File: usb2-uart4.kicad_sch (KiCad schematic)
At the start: 14 parts, among them U1 FT4232H, U2 NUP2202, U3 93LCxxB, Y1 12.000 MHz

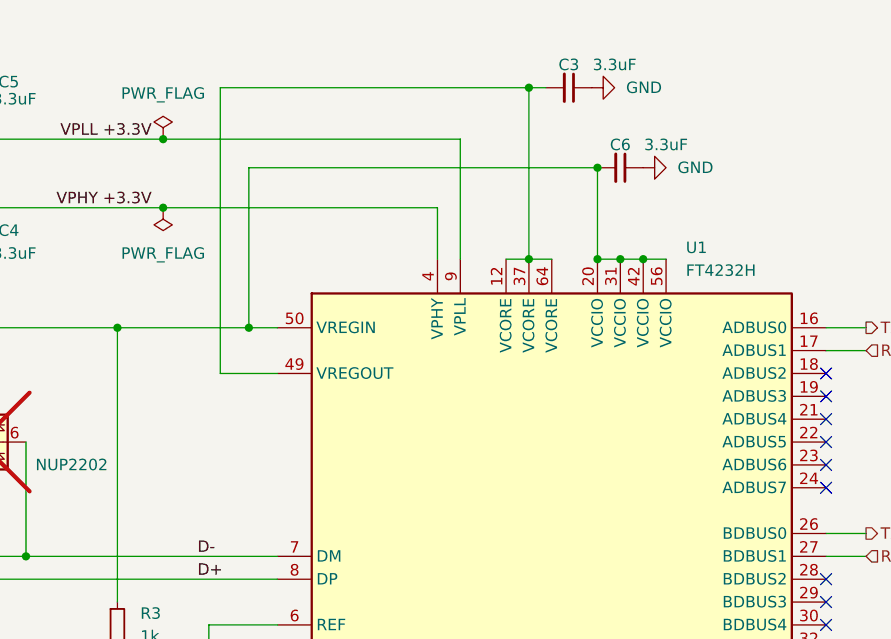
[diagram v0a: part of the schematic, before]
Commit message: Flush
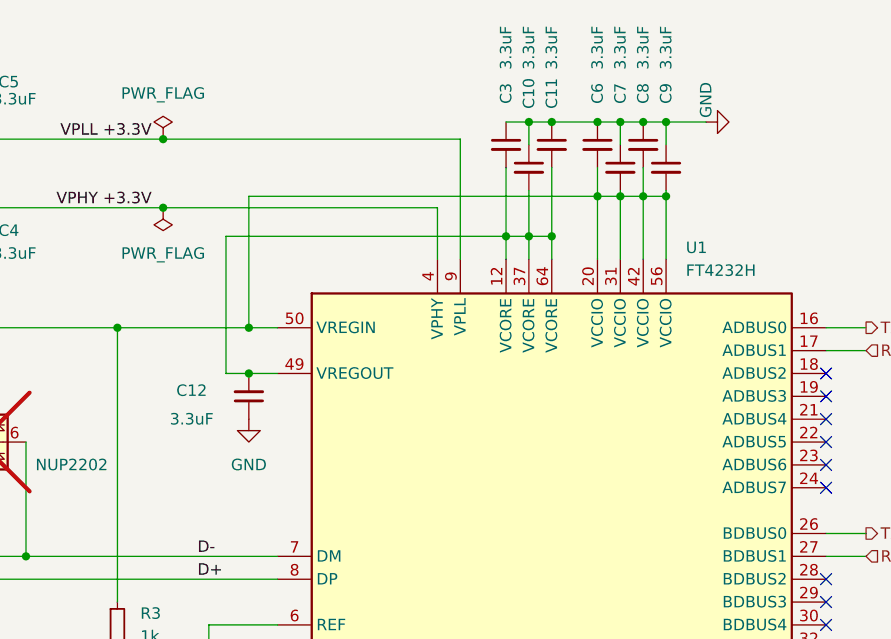
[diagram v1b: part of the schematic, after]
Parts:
- added C10, C11, C12, C7, C8, C9: 3.3uF, Capacitor_SMD:C_0805_2012Metric_Pad1.18x1.45mm_HandSolder, symbol Device:C_Small
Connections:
- net GND: now also C10.1, C11.1, C12.1, C7.1, C8.1, C9.1
- net VIN 3.3V: now also C7.2, C8.2, C9.2
- net at C3.2, U1.12 (VCORE), U1.37 (VCORE)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: now also C10.2, C11.2, C12.2
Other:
- moved on the sheet: C3, C6
